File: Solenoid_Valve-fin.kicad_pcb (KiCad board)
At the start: 2 copper layers, 85.9 x 100 mm, 118 parts, among them IC1 Si8621AB-B-ISR, J1 Bus_mechaken_PCIexpress_x16_1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, J10 Conn_01x02, J11 Conn_01x02, J12 Conn_01x02, J13 Conn_01x02, J14 Conn_01x02, J15 Conn_01x02, J16 Conn_01x02, J17 Conn_01x02, J18 Conn_01x02, J19 Conn_01x02, J2 Conn_01x05, J20 Conn_01x02, J3 Conn_01x02, J4 Conn_01x02, J5 Conn_01x02, J6 Conn_01x02, J7 Conn_01x03, J8 Conn_01x02, J9 Conn_01x02, Q1 ULN2004D1013TR, Q2 ULN2004D1013TR, Q3 ULN2004D1013TR, U1 LDL1117S33R, U2 STM32F042K6Tx, U3 MCP2562-E-SN, U4 L7812, U5 LDL1117S33R

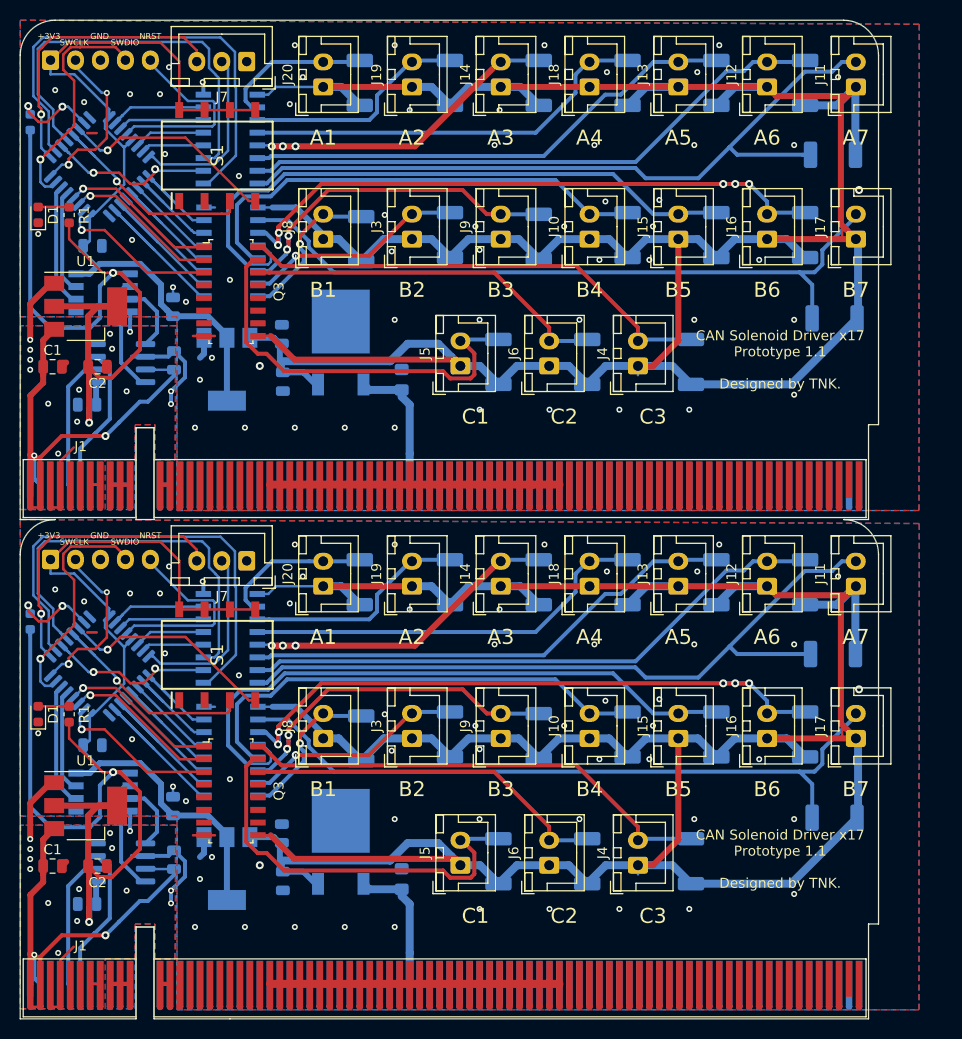
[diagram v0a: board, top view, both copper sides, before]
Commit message: Release
ガーバーファイルを出力
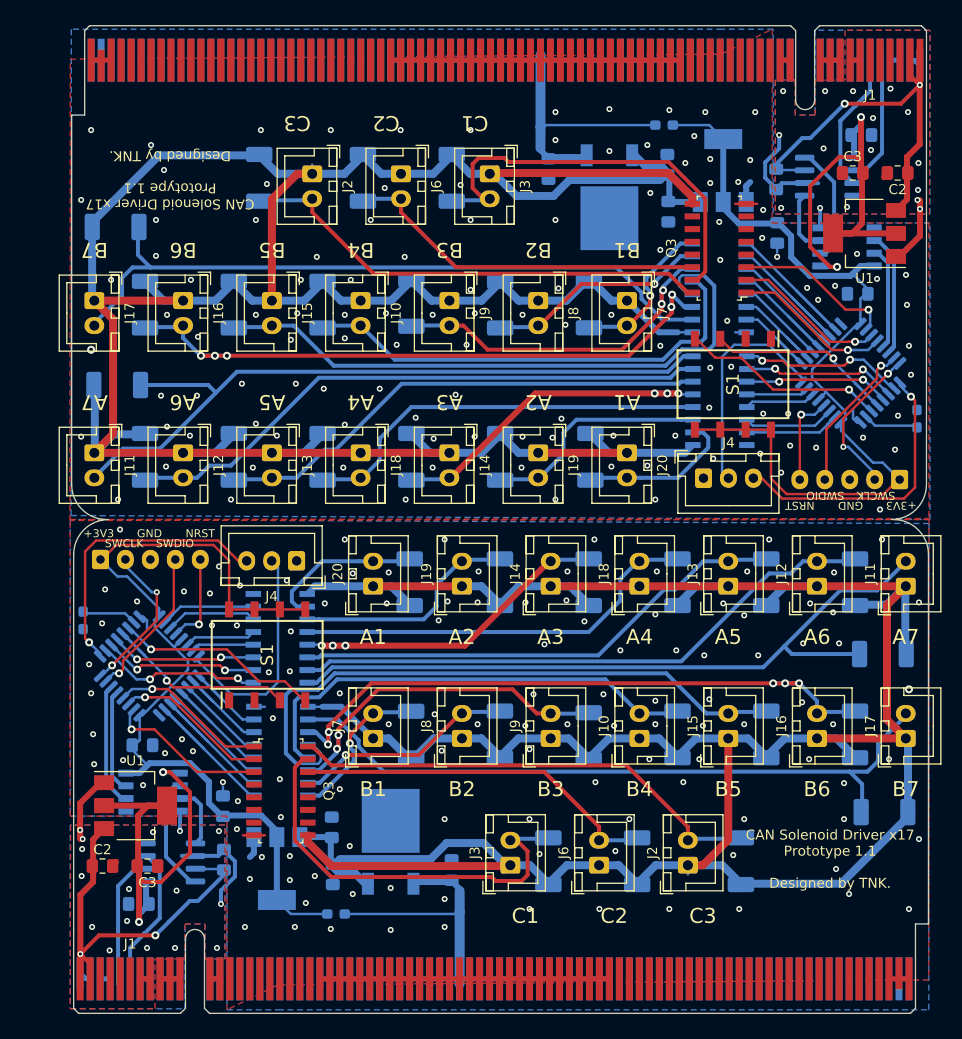
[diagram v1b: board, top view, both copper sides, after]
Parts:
- removed C10: 4.7uF, Capacitor_SMD:C_0805_2012Metric
- removed the D1 at (121.8, 49.5)
- removed the D1 at (121.8, 99.5)
- removed the D18 at (163.0, 36.3)
- removed D19: D, Diode_SMD:D_2010_5025Metric
- removed the R1 at (124.9, 49.5)
- removed the R1 at (124.9, 99.5)
- removed R2: 10K, Resistor_SMD:R_0603_1608Metric
- added C3: 4.7uF, Capacitor_SMD:C_0805_2012Metric_Pad1.15x1.40mm_HandSolder, F.Cu at (203.4, 45.3)
- added D1: D, Diode_SMD:D_2010_5025Metric_Pad1.52x2.65mm_HandSolder, B.Cu at (143.9, 45.8)
- added D18: D_Schottky, Diode_SMD:D_0603_1608Metric_Pad1.05x0.95mm_HandSolder, B.Cu at (184.5, 40.5)
- added D18: D_Schottky, Diode_SMD:D_0603_1608Metric_Pad1.05x0.95mm_HandSolder, B.Cu at (151.6, 119.5)
- added D5: D, Diode_SMD:D_2010_5025Metric_Pad1.52x2.65mm_HandSolder, B.Cu at (168.1, 58.5)
- added R1: 10K, Resistor_SMD:R_0603_1608Metric_Pad1.05x0.95mm_HandSolder, B.Cu at (209.8, 69.9)
- C1: value 1.0uF -> 0.1uF; footprint Capacitor_SMD:C_0805_2012Metric -> Capacitor_SMD:C_0805_2012Metric_Pad1.15x1.40mm_HandSolder; moved to B.Cu
- C1: renamed from C5; footprint Capacitor_SMD:C_0805_2012Metric -> Capacitor_SMD:C_0805_2012Metric_Pad1.15x1.40mm_HandSolder
- C2: value 4.7uF -> 1.0uF; footprint Capacitor_SMD:C_0805_2012Metric -> Capacitor_SMD:C_0805_2012Metric_Pad1.15x1.40mm_HandSolder
- C2: renamed from C1; footprint Capacitor_SMD:C_0805_2012Metric -> Capacitor_SMD:C_0805_2012Metric_Pad1.15x1.40mm_HandSolder
- C3: renamed from C2; footprint Capacitor_SMD:C_0805_2012Metric -> Capacitor_SMD:C_0805_2012Metric_Pad1.15x1.40mm_HandSolder
- C4, C6: footprint Capacitor_SMD:C_0805_2012Metric -> Capacitor_SMD:C_0805_2012Metric_Pad1.15x1.40mm_HandSolder
- C4: renamed from C6; footprint Capacitor_SMD:C_0805_2012Metric -> Capacitor_SMD:C_0805_2012Metric_Pad1.15x1.40mm_HandSolder
- C5: value 0.1uF -> 1.0uF; footprint Capacitor_SMD:C_0805_2012Metric -> Capacitor_SMD:C_0805_2012Metric_Pad1.15x1.40mm_HandSolder
- C5: renamed from C9; footprint Capacitor_SMD:C_0805_2012Metric -> Capacitor_SMD:C_0805_2012Metric_Pad1.15x1.40mm_HandSolder
- C6: renamed from C4; footprint Capacitor_SMD:C_0805_2012Metric -> Capacitor_SMD:C_0805_2012Metric_Pad1.15x1.40mm_HandSolder
- C7: value 1uF -> 4.7uF
- C7: renamed from C10; footprint Capacitor_SMD:C_0805_2012Metric -> Capacitor_SMD:C_0805_2012Metric_Pad1.15x1.40mm_HandSolder
- C8: value 4.7uF -> 0.33uF; footprint Capacitor_SMD:C_0805_2012Metric -> Capacitor_SMD:C_0805_2012Metric_Pad1.15x1.40mm_HandSolder
- C8: renamed from C7; value 1uF -> 0.33uF
- C9: value 1.0uF -> 0.1uF; footprint Capacitor_SMD:C_0805_2012Metric -> Capacitor_SMD:C_0805_2012Metric_Pad1.15x1.40mm_HandSolder
- C9: renamed from C8; value 4.7uF -> 0.1uF; footprint Capacitor_SMD:C_0805_2012Metric -> Capacitor_SMD:C_0805_2012Metric_Pad1.15x1.40mm_HandSolder
- D1: renamed from D2; footprint Diode_SMD:D_2010_5025Metric -> Diode_SMD:D_2010_5025Metric_Pad1.52x2.65mm_HandSolder
- D10, D11, D12, D13, D14, D15, D16, D17, D2, D3, D4, D6, D7, D8, D9: footprint Diode_SMD:D_2010_5025Metric -> Diode_SMD:D_2010_5025Metric_Pad1.52x2.65mm_HandSolder
- D10: renamed from D12; footprint Diode_SMD:D_2010_5025Metric -> Diode_SMD:D_2010_5025Metric_Pad1.52x2.65mm_HandSolder
- D11: renamed from D13; footprint Diode_SMD:D_2010_5025Metric -> Diode_SMD:D_2010_5025Metric_Pad1.52x2.65mm_HandSolder
- D12: renamed from D14; footprint Diode_SMD:D_2010_5025Metric -> Diode_SMD:D_2010_5025Metric_Pad1.52x2.65mm_HandSolder
- D13: renamed from D15; footprint Diode_SMD:D_2010_5025Metric -> Diode_SMD:D_2010_5025Metric_Pad1.52x2.65mm_HandSolder
- D14: renamed from D16; footprint Diode_SMD:D_2010_5025Metric -> Diode_SMD:D_2010_5025Metric_Pad1.52x2.65mm_HandSolder
- D15: renamed from D17; footprint Diode_SMD:D_2010_5025Metric -> Diode_SMD:D_2010_5025Metric_Pad1.52x2.65mm_HandSolder
- D16: renamed from D18; footprint Diode_SMD:D_2010_5025Metric -> Diode_SMD:D_2010_5025Metric_Pad1.52x2.65mm_HandSolder
- D17: renamed from D19; footprint Diode_SMD:D_2010_5025Metric -> Diode_SMD:D_2010_5025Metric_Pad1.52x2.65mm_HandSolder
- D2: renamed from D3; footprint Diode_SMD:D_2010_5025Metric -> Diode_SMD:D_2010_5025Metric_Pad1.52x2.65mm_HandSolder
- D3: renamed from D4; footprint Diode_SMD:D_2010_5025Metric -> Diode_SMD:D_2010_5025Metric_Pad1.52x2.65mm_HandSolder
- D4: renamed from D6; footprint Diode_SMD:D_2010_5025Metric -> Diode_SMD:D_2010_5025Metric_Pad1.52x2.65mm_HandSolder
- D5: renamed from D7; footprint Diode_SMD:D_2010_5025Metric -> Diode_SMD:D_2010_5025Metric_Pad1.52x2.65mm_HandSolder
- D6: renamed from D8; footprint Diode_SMD:D_2010_5025Metric -> Diode_SMD:D_2010_5025Metric_Pad1.52x2.65mm_HandSolder
- D7: renamed from D9; footprint Diode_SMD:D_2010_5025Metric -> Diode_SMD:D_2010_5025Metric_Pad1.52x2.65mm_HandSolder
- D8: renamed from D10; footprint Diode_SMD:D_2010_5025Metric -> Diode_SMD:D_2010_5025Metric_Pad1.52x2.65mm_HandSolder
- D9: renamed from D11; footprint Diode_SMD:D_2010_5025Metric -> Diode_SMD:D_2010_5025Metric_Pad1.52x2.65mm_HandSolder
- J1 (x2): footprint PCIe:BUS_mechaken_PCIexpress_x16_164_Position -> PCIe:BUS_mechaken_PCIexpress_x16
- J2: value Conn_01x05 -> Conn_01x02; footprint Connector_JST:JST_XH_B5B-XH-A_1x05_P2.50mm_Vertical -> Connector_JST:JST_XH_B2B-XH-A_1x02_P2.50mm_Vertical; moved to F.Cu
- J4: value Conn_01x02 -> Conn_01x03; footprint Connector_JST:JST_XH_B2B-XH-A_1x02_P2.50mm_Vertical -> Connector_JST:JST_XH_B3B-XH-A_1x03_P2.50mm_Vertical
- J5: value Conn_01x02 -> Conn_01x05; footprint Connector_JST:JST_XH_B2B-XH-A_1x02_P2.50mm_Vertical -> Connector_JST:JST_XH_B5B-XH-A_1x05_P2.50mm_Vertical; moved to B.Cu
- J7: value Conn_01x03 -> Conn_01x02; footprint Connector_JST:JST_XH_B3B-XH-A_1x03_P2.50mm_Vertical -> Connector_JST:JST_XH_B2B-XH-A_1x02_P2.50mm_Vertical
- R1: renamed from R2; footprint Resistor_SMD:R_0603_1608Metric -> Resistor_SMD:R_0603_1608Metric_Pad1.05x0.95mm_HandSolder
- U2: value STM32F042K6Tx -> MCP2562-E-SN; footprint Package_QFP:LQFP-32_7x7mm_P0.8mm -> Package_SO:SOIC-8_3.9x4.9mm_P1.27mm
- U3: value MCP2562-E-SN -> STM32F042K6Tx; footprint Package_SO:SOIC-8_3.9x4.9mm_P1.27mm -> Package_QFP:LQFP-32_7x7mm_P0.8mm
- U4: value L7812 -> LDL1117S33R; footprint Package_TO_SOT_SMD:TO-252-2 -> Package_TO_SOT_SMD:SOT-223-3_TabPin2
- U5: value LDL1117S33R -> NJM7812; footprint Package_TO_SOT_SMD:SOT-223-3_TabPin2 -> Package_TO_SOT_SMD:TO-252-2
- U5: renamed from U4; value L7812 -> NJM7812
- moved J1 98.5 mm to (210.1, 34.0), turned to 180 degrees
- moved J11 84.6 mm to (127.4, 73.3), turned to 270 degrees
- moved C1 84.2 mm to (204.2, 41.5), turned to 180 degrees
- moved C2 82.4 mm to (207.9, 45.3)
- moved U1 78.3 mm to (204.6, 51.4), turned to 180 degrees
- moved J17 76.5 mm to (127.4, 58.1), turned to 270 degrees
- moved IC1 74.6 mm to (202.8, 52.7), turned to 0 degrees
- moved U3 73.1 mm to (203.2, 65.3), turned to 45 degrees
- moved U2 73.1 mm to (201.0, 45.7), turned to 0 degrees
- moved J12 69.0 mm to (136.3, 73.3), turned to 270 degrees
- moved C4 68.8 mm to (195.7, 45.9), turned to 90 degrees
- moved C6 68.8 mm to (203.9, 57.4), turned to 0 degrees
- moved D10 67.2 mm to (141.4, 73.7), turned to 270 degrees
- moved C5 61.3 mm to (184.9, 49.2), turned to 270 degrees
- moved D14 60.2 mm to (129.6, 50.7), turned to 0 degrees
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- renumbered J4 to J2, J5 to J3, J7 to J4, J2 to J5, J8 to J7, J3 to J8, U3 to U2, U2 to U3, U5 to U4
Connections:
- C1 pad 1: +5V -> GND
- C1 pad 2: GND -> +3V3
- C2 pad 1: GND -> +5V
- C2 pad 2: +3V3 -> GND
- C4 pad 1: GNDPWR -> GND
- C4 pad 2: 3.3V -> +5V
- C5 pad 1: GND -> +12V
- C5 pad 2: +3V3 -> GNDPWR
- C6 pad 1: GND -> GNDPWR
- C6 pad 2: +5V -> 3.3V
- C7 pad 1: VCC -> 3.3V
- C8 pad 1: +12V -> VCC
- D10 pad 2: Solenoid_B1 -> Solenoid_B3
- D11 pad 2: Solenoid_B2 -> Solenoid_B4
- D12 pad 2: Solenoid_B3 -> Solenoid_A5
- D13 pad 2: Solenoid_B4 -> Solenoid_A6
- D14 pad 2: Solenoid_A5 -> Solenoid_A7
- D15 pad 2: Solenoid_A6 -> Solenoid_B5
- D16 pad 2: Solenoid_A7 -> Solenoid_B6
- D17 pad 2: Solenoid_B5 -> Solenoid_B7
- D2 pad 2: Solenoid_C1 -> Solenoid_C2
- D3 pad 2: Solenoid_C2 -> Solenoid_C3
- D4 pad 2: Solenoid_C3 -> Solenoid_A1
- D6 pad 2: Solenoid_A1 -> Solenoid_A3
- D7 pad 2: Solenoid_A2 -> Solenoid_A4
- D8 pad 2: Solenoid_A3 -> Solenoid_B1
- D9 pad 2: Solenoid_A4 -> Solenoid_B2
- J2 pad 1: 3.3V -> +12V
- J2 pad 2: /SWCLK -> Solenoid_C1
- J3 pad 2: Solenoid_A2 -> Solenoid_C2
- J4 pad 1: +12V -> GNDPWR
- J4 pad 2: Solenoid_C1 -> VCP_TX
- J5 pad 1: +12V -> 3.3V
- J5 pad 2: Solenoid_C2 -> /SWCLK
- J7 pad 1: GNDPWR -> +12V
- J7 pad 2: VCP_TX -> Solenoid_A1
- J8 pad 2: Solenoid_A1 -> Solenoid_A2
- Q3 pad 10: (no net) -> Net-(Q3-Pad10) (x2)
- Q3 pad 11: (no net) -> Net-(Q3-Pad11) (x2)
- Q3 pad 12: (no net) -> Net-(Q3-Pad12) (x2)
- Q3 pad 13: (no net) -> Net-(Q3-Pad13) (x2)
- Q3 pad 4: (no net) -> Net-(Q3-Pad4) (x2)
- Q3 pad 5: (no net) -> Net-(Q3-Pad5) (x2)
- Q3 pad 6: (no net) -> Net-(Q3-Pad6) (x2)
- Q3 pad 7: (no net) -> Net-(Q3-Pad7) (x2)
- R1 pad 2: +3V3 -> GNDPWR
- S1 pad 1: (no net) -> Net-(S1-Pad1) (x2)
- S1 pad 2: (no net) -> Net-(S1-Pad2) (x2)
- U2 pad 1: 3.3V -> CAN_TXD
- U2 pad 2: IC_B7 -> GND
- U2 pad 3: IC_B6 -> +5V
- U2 pad 4: NRST -> CAN_RXD
- U2 pad 5: 3.3V -> +3V3
- U2 pad 6: IC_B5 -> CAN-
- U2 pad 7: IC_B4 -> CAN+
- U2 pad 8: VCP_TX -> GND
- U3 pad 1: CAN_TXD -> 3.3V
- U3 pad 2: GND -> IC_B7
- U3 pad 3: +5V -> IC_B6
- U3 pad 4: CAN_RXD -> NRST
- U3 pad 5: +3V3 -> 3.3V
- U3 pad 6: CAN- -> IC_B5
- U3 pad 7: CAN+ -> IC_B4
- U3 pad 8: GND -> VCP_TX
- U4 pad 1: VCC -> GNDPWR
- U4 pad 2: GNDPWR -> 3.3V
- U5 pad 1: GNDPWR -> VCC
- U5 pad 2: 3.3V -> GNDPWR
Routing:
- net +12V: track 733.2 -> 627.9 mm
- net +3V3: track 164.7 -> 90.8 mm
- net IC_B1: track 94.8 -> 34.2 mm, vias 0 -> 4
- net IC_B3: track 83.3 -> 29.2 mm, vias 0 -> 4
- net +5V: track 117.1 -> 92.9 mm
- net NRST: track 40.6 -> 20.2 mm, vias 0 -> 2
- net VCC: track 90.8 -> 110.6 mm
- net /SWDIO: track 47.6 -> 30.8 mm
- net GND: track 54.3 -> 43.2 mm, vias 28 -> 32
- net VCP_TX: track 36.0 -> 45.5 mm
- net 3.3V: track 168.2 -> 177.6 mm
- net Net-(J1-PadB5): track 11.2 -> 2.00 mm
- net Net-(J1-PadA5): track 11.2 -> 2.00 mm
- net Net-(D1-Pad2): track 6.21 -> 0.00 mm
- net /BOOT: track 17.7 -> 11.5 mm, vias 4 -> 0
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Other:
- board size 85.9 x 100 mm -> 85.8 x 82.1 mm
